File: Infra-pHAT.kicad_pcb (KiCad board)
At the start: 2 copper layers, 65 x 30 mm, 25 parts, among them Q1 BC817, U1 CAT24C32WI-GT3

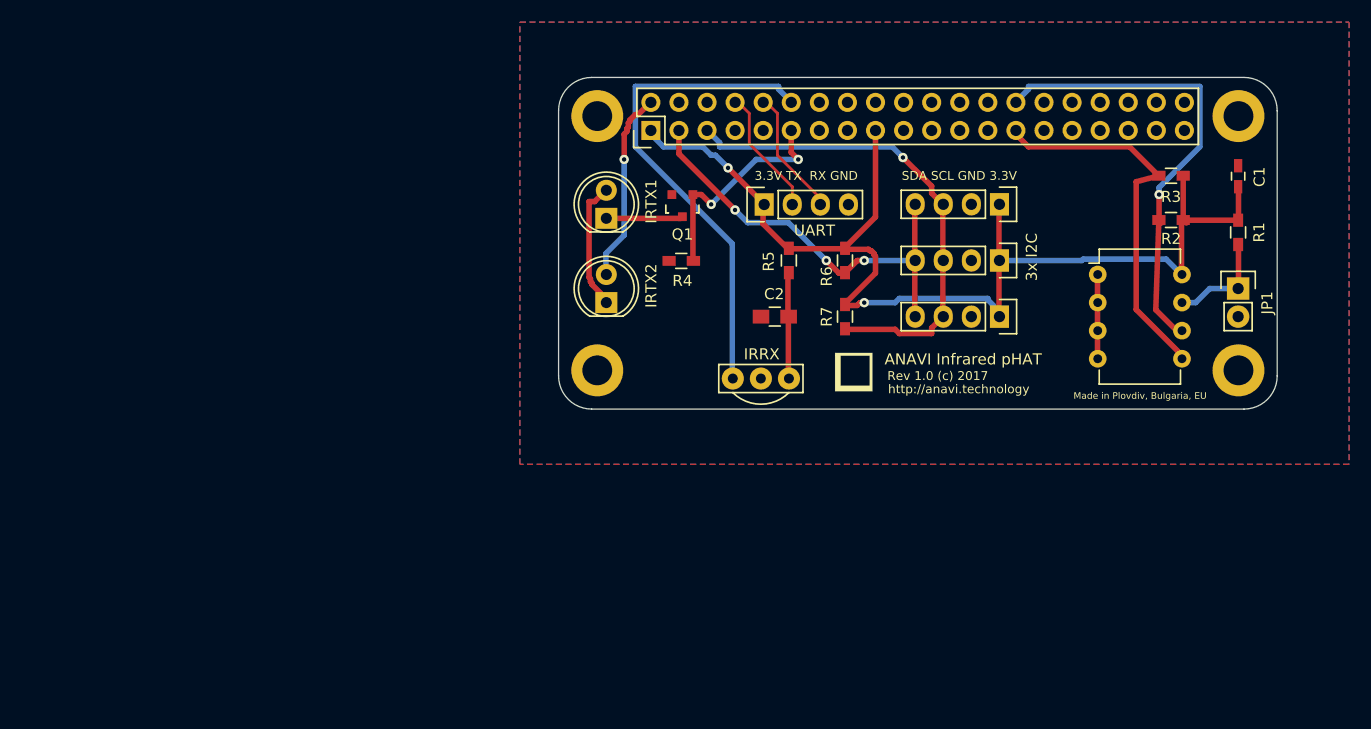
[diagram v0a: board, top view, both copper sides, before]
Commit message: Initial version SCH + PCM
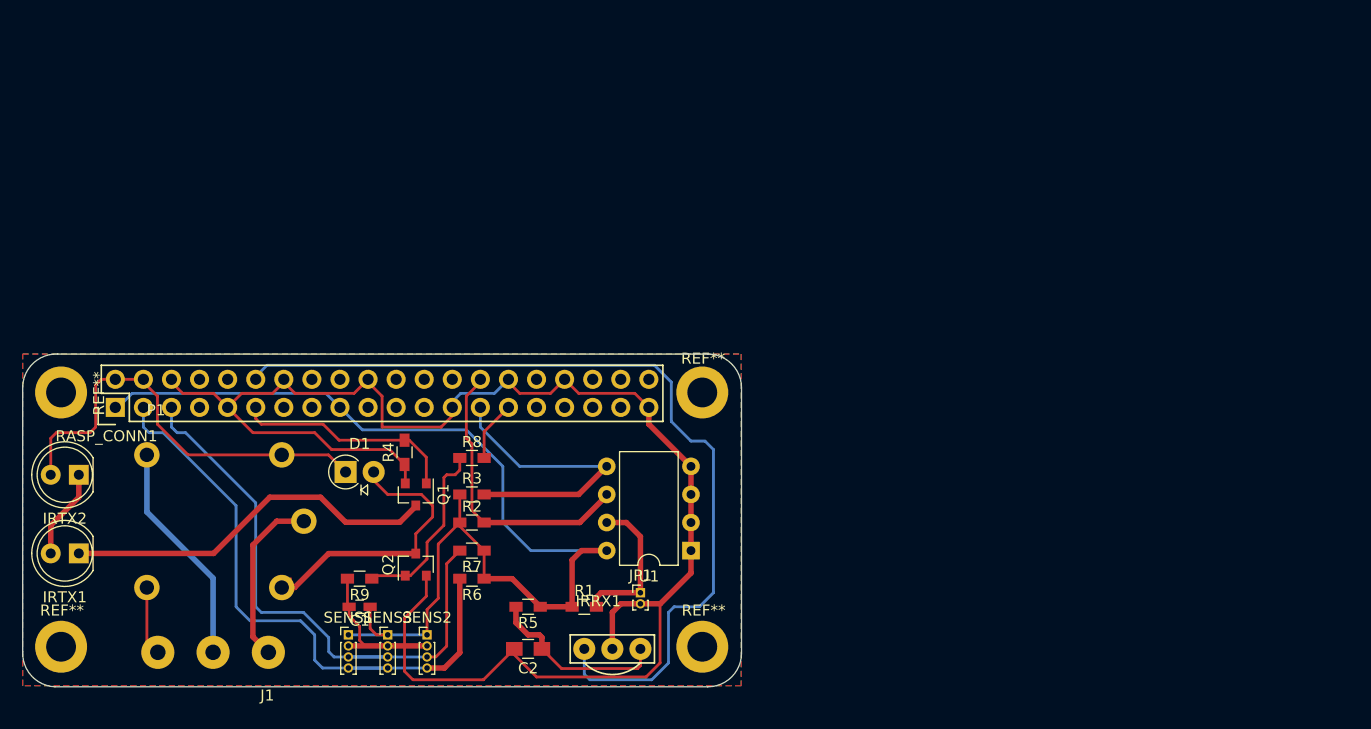
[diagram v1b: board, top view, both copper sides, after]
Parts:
- removed ?: LOGO, logo:anavi-logo
- removed IRRX: TSOP34838, myfootprint:TSOP38X
- removed REF1, REF2, REF3, REF4: MountingHole_2.7mm_M2.5_DIN965_Pad, Mounting_Holes:MountingHole_2.7mm_M2.5_DIN965_Pad
- removed UART: CONN_01X04, Pin_Headers:Pin_Header_Straight_1x04
- added D1: 1N4148, Diodes_THT:D_T-1_P2.54mm_Vertical_AnodeUp, F.Cu at (129.2, 110.7)
- added IRRX1: TSOP34838, myfootprint:TSOP38X, F.Cu at (153.4, 124.2)
- added J1: CONN_01X03, myfootprint:KLEMA_1x3, F.Cu at (122.3, 130.5)
- added P1: RAS-05-15, myfootprint:RAS-05-15, F.Cu at (113.4, 107.6)
- added Q2: BC817-40, TO_SOT_Packages_SMD:SOT-23, F.Cu at (135.6, 119.1)
- added R8: 2.7k, Resistors_SMD:R_0603_HandSoldering, F.Cu at (140.7, 109.4)
- added R9: 27k, Resistors_SMD:R_0603_HandSoldering, F.Cu at (130.5, 120.3)
- added REF**: MountingHole_2.7mm_M2.5_DIN965_Pad, Mounting_Holes:MountingHole_2.7mm_M2.5_DIN965_Pad, F.Cu at (161.6, 103.8)
- added REF**: MountingHole_2.7mm_M2.5_DIN965_Pad, Mounting_Holes:MountingHole_2.7mm_M2.5_DIN965_Pad, F.Cu at (103.6, 103.6)
- added REF**: MountingHole_2.7mm_M2.5_DIN965_Pad, Mounting_Holes:MountingHole_2.7mm_M2.5_DIN965_Pad, F.Cu at (161.6, 126.6)
- added REF**: MountingHole_2.7mm_M2.5_DIN965_Pad, Mounting_Holes:MountingHole_2.7mm_M2.5_DIN965_Pad, F.Cu at (103.6, 126.6)
- IRTX1, IRTX2: footprint LEDs:LED-5MM -> LEDs:LED_D5.0mm
- JP1: footprint Pin_Headers:Pin_Header_Straight_1x02 -> Pin_Headers:Pin_Header_Straight_1x02_Pitch1.00mm
- RASP_CONN1: footprint Pin_Headers:Pin_Header_Straight_2x20 -> myfootprint:Pin_Header_Straight_2x20
- SENS1, SENS2, SENS3: footprint Pin_Headers:Pin_Header_Straight_1x04 -> Pin_Headers:Pin_Header_Straight_1x04_Pitch1.00mm
- moved C1 88.5 mm to (130.5, 122.9), turned to 180 degrees
- moved R3 69.5 mm to (140.7, 112.7), turned to 0 degrees
- moved R2 68.9 mm to (140.7, 115.3), turned to 0 degrees
- moved R1 68.2 mm to (150.8, 122.9), turned to 0 degrees
- moved SENS3 67.7 mm to (133.0, 125.4), turned to 0 degrees
- moved SENS1 65.5 mm to (129.5, 125.4), turned to 0 degrees
- moved SENS2 61.9 mm to (136.6, 125.4), turned to 0 degrees
- moved JP1 60.7 mm to (155.9, 121.6)
- moved IRTX1 56.5 mm to (105.1, 118.1), turned to 180 degrees
- moved IRTX2 50.2 mm to (105.1, 110.9), turned to 180 degrees
- moved U1 44.5 mm to (160.5, 117.8), turned to 180 degrees
- moved R6 44.4 mm to (140.7, 120.3), turned to 180 degrees
- moved R7 39.8 mm to (140.7, 117.8), turned to 180 degrees
- moved R5 39.2 mm to (145.7, 122.9), turned to 180 degrees
- moved C2 37.4 mm to (145.7, 126.7)
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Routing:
- net GND: track 8.40 -> 181.3 mm
- net Net-(IRTX1-Pad1): track 7.02 -> 56.2 mm
- net Net-(IRRX1-Pad1): track 45.1 -> 80.4 mm
- net Net-(D1-Pad2): track 0.00 -> 26.5 mm
- net +5V: track 17.5 -> 40.4 mm, vias 1 -> 0
- net Net-(J1-Pad2): track 0.00 -> 20.3 mm
- net Net-(R6-Pad2): track 39.0 -> 56.9 mm, vias 3 -> 0
- net Net-(Q2-Pad1): track 0.00 -> 16.6 mm
- net Net-(J1-Pad1): track 0.00 -> 15.8 mm
- net /RXD: track 11.6 -> 0.00 mm
- net /TXD: track 11.6 -> 0.00 mm
- net Net-(JP1-Pad1): track 10.1 -> 21.4 mm
- net Net-(R7-Pad2): track 45.2 -> 54.7 mm, vias 1 -> 0
- net Net-(R3-Pad2): track 35.1 -> 26.8 mm
- net Net-(C2-Pad1): track 9.96 -> 16.9 mm
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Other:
- board size 65 x 30 mm -> 65 x 30.1 mm
- net class vcc removed
- rule trace_min: 0.25 -> 0.254
- rule via_min_drill: 0.3 -> 0.35
- rule via_min_size: 0.4 -> 0.7
- board text removed: "100nF"
- board text removed: "10K"
- board text removed: "1K"
- board text removed: "3.3V TX RX GND"
- board text removed: "3x I2C"
- board text removed: "4,7K"
- board text removed: "4,7pF"
- board text removed: "470"
- board text removed: "ANAVI Infrared pHAT"
- board text removed: "BC817"
- board text removed: "Made in Plovdiv, Bulgaria, EU"
- board text removed: "Rev 1.0 (c) 2017"
- board text removed: "SDA SCL GND 3.3V"
- board text removed: "http://anavi.technology"
